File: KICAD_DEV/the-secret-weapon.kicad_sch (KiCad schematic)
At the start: 7 parts, among them J1 USB_C_Receptacle_USB2.0_14P, U1 STM32H757IITx, U2 TPS26750

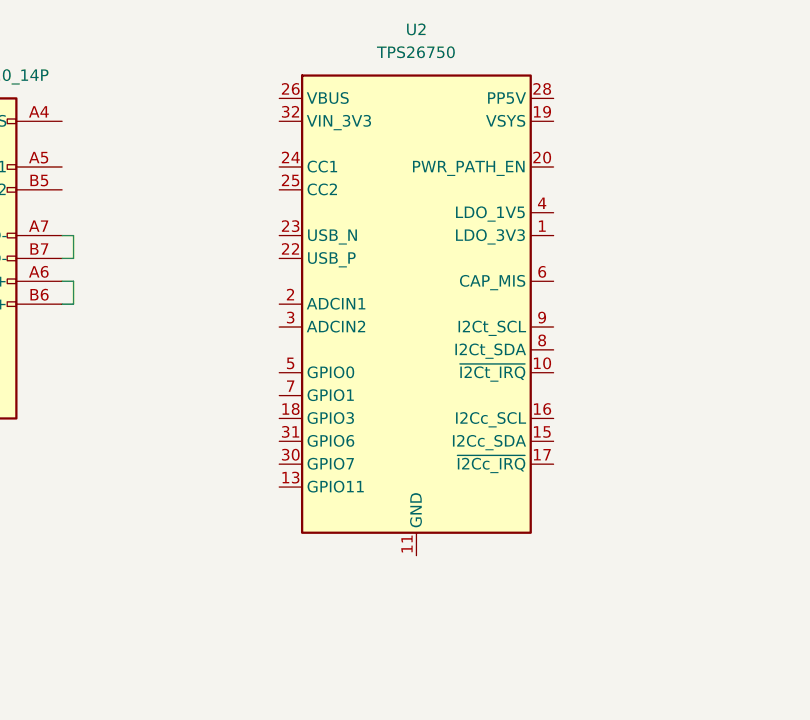
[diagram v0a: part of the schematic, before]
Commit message: revising my USB PD
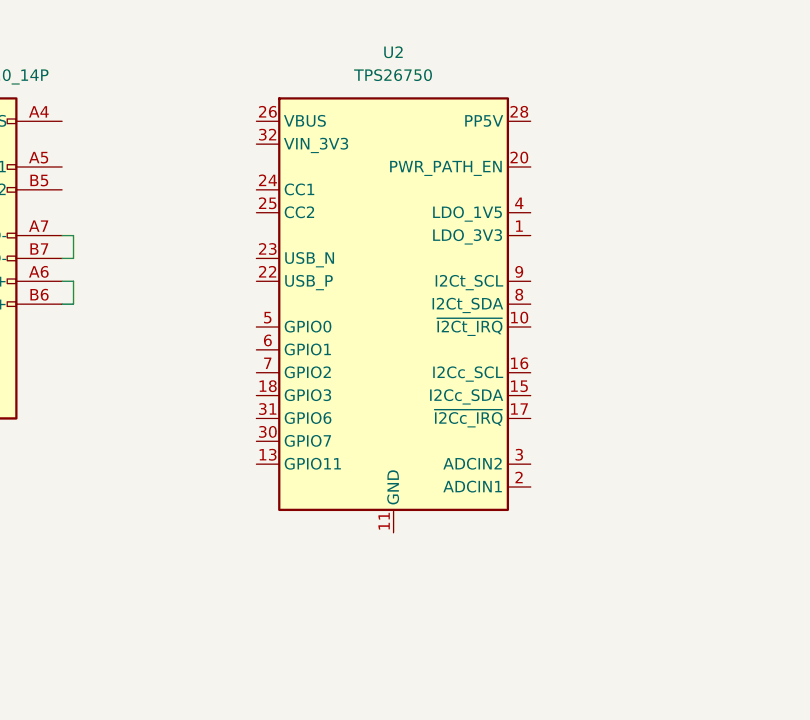
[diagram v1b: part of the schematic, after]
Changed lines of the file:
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@@
+	)
+	(symbol
+		(lib_id "kai-library:TPS26750")
+		(at 166.37 66.04 0)
+		(unit 1)
+		(exclude_from_sim no)
+		(in_bom yes)
+		(on_board yes)
+		(dnp no)
+		(fields_autoplaced yes)
+		(property "Reference" "U2"
+			(at 166.37 43.18 0)
+			(effects
+				(font
+					(size 1.27 1.27)
+				)
+			)
+		)
+		(property "Value" "TPS26750"
+			(at 166.37 45.72 0)
+			(effects
+				(font
+					(size 1.27 1.27)
+				)
+			)
+		)
+		(property "Footprint" "Package_DFN_QFN:Texas_RSN_WQFN-32-1EP_4x4mm_P0.4mm_EP2.8x2.8mm_ThermalVias"
+			(at 166.37 66.04 0)
+			(effects
+				(font
+					(size 1.27 1.27)
+				)
+				(hide yes)
+			)
+		)
+		(property "Datasheet" "https://www.ti.com/lit/ds/symlink/tps26750.pdf?ts=1761278028610&ref_url=https%253A%252F%252Fwww.ti.com%252Fproduct%252FTPS26750"
+			(at 166.37 66.04 0)
+			(effects
+				(font
+					(size 1.27 1.27)
+				)
+				(hide yes)
+			)
+		)
+		(property "Description" "TPS26750 USB Type-C® and USB PD Controller With Integrated Power Switches Optimized for Power Applications"
+			(at 166.37 66.04 0)
+			(effects
+				(font
+					(size 1.27 1.27)
+				)
+				(hide yes)
+			)
+		)
+		(pin "30"
+		)
+		(pin "31"
+		)
+		(pin "12"
+		)
+		(pin "34"
+		)
+		(pin "3"
+		)
+		(pin "20"
+		)
+		(pin "22"
+		)
+		(pin "10"
+		)
+		(pin "16"
+		)
+		(pin "31"
+		)
+		(pin "13"
+		)
+		(pin "39"
+		)
+		(pin "9"
+		)
+		(pin "16"
+		)
+		(pin "23"
+		)
+		(pin "1"
+		)
+		(pin "17"
+		)
+		(pin "2"
+		)
+		(pin "14"
+		)
+		(pin "7"
+		)
+		(pin "15"
+		)
+		(pin "5"
+		)
+		(pin "11"
+		)
+		(pin "8"
+		)
+		(pin "32"
+		)
+		(pin "26"
+		)
+		(pin "18"
+		)
+		(pin "6"
+		)
+		(pin "24"
+		)
+		(pin "25"
+		)
+		(pin "4"
+		)
+		(pin "17"
+		)
+		(pin "28"
+		)
+		(instances
+			(project ""
+				(path "/28389848-e686-45d1-8788-e912d76b51d3"
+					(reference "U2")
+					(unit 1)
+				)
+			)
+		)
 	)
 	(symbol
@@
 					(unit 1)
 				)
-			)
-		)
-	)
-	(symbol
-		(lib_id "kai-library:TPS26750")
-		(at 168.91 63.5 0)
-		(unit 1)
-		(exclude_from_sim no)
-		(in_bom yes)
-		(on_board yes)
-		(dnp no)
-		(fields_autoplaced yes)
-		(property "Reference" "U2"
-			(at 168.91 40.64 0)
-			(effects
-				(font
-					(size 1.27 1.27)
-				)
-			)
-		)
-		(property "Value" "TPS26750"
-			(at 168.91 43.18 0)
-			(effects
-				(font
-					(size 1.27 1.27)
-				)
-			)
-		)
-		(property "Footprint" "Package_DFN_QFN:Texas_RSN_WQFN-32-1EP_4x4mm_P0.4mm_EP2.8x2.8mm_ThermalVias"
-			(at 168.91 63.5 0)
-			(effects
-				(font
-					(size 1.27 1.27)
-				)
-				(hide yes)
-			)
-		)
-		(property "Datasheet" "https://www.ti.com/lit/ds/symlink/tps26750.pdf?ts=1761278028610&ref_url=https%253A%252F%252Fwww.ti.com%252Fproduct%252FTPS26750"
-			(at 168.91 63.5 0)
-			(effects
-				(font
-					(size 1.27 1.27)
-				)
-				(hide yes)
-			)
-		)
-		(property "Description" "TPS26750 USB Type-C® and USB PD Controller With Integrated Power Switches Optimized for Power Applications"
-			(at 168.91 63.5 0)
-			(effects
-				(font
-					(size 1.27 1.27)
-				)
-				(hide yes)
-			)
-		)
-		(pin "6"
-		)
-		(pin "5"
-		)
-		(pin "13"
-		)
-		(pin "12"
-		)
-		(pin "25"
-		)
-		(pin "24"
-		)
-		(pin "1"
-		)
-		(pin "18"
-		)
-		(pin "14"
-		)
-		(pin "10"
-		)
-		(pin "34"
-		)
-		(pin "26"
-		)
-		(pin "16"
-		)
-		(pin "17"
-		)
-		(pin "9"
-		)
-		(pin "16"
-		)
-		(pin "15"
-		)
-		(pin "8"
-		)
-		(pin "28"
-		)
-		(pin "39"
-		)
-		(pin "11"
-		)
-		(pin "22"
-		)
-		(pin "17"
-		)
-		(pin "30"
-		)
-		(pin "23"
-		)
-		(pin "19"
-		)
-		(pin "7"
-		)
-		(pin "32"
-		)
-		(pin "31"
-		)
-		(pin "2"
-		)
-		(pin "20"
-		)
-		(pin "4"
-		)
-		(pin "31"
-		)
-		(pin "3"
-		)
-		(instances
-			(project ""
-				(path "/28389848-e686-45d1-8788-e912d76b51d3"
-					(reference "U2")
-					(unit 1)
-				)
